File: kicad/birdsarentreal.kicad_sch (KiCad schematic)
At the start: 31 parts, among them J1 Adafruit Coil Jumper, J2 Adafruit Coil Jumper, J3 Adafruit Coil Jumper, J4 Adafruit Coil Jumper, Q2 NMOS, U9 MCP73831-2-OT

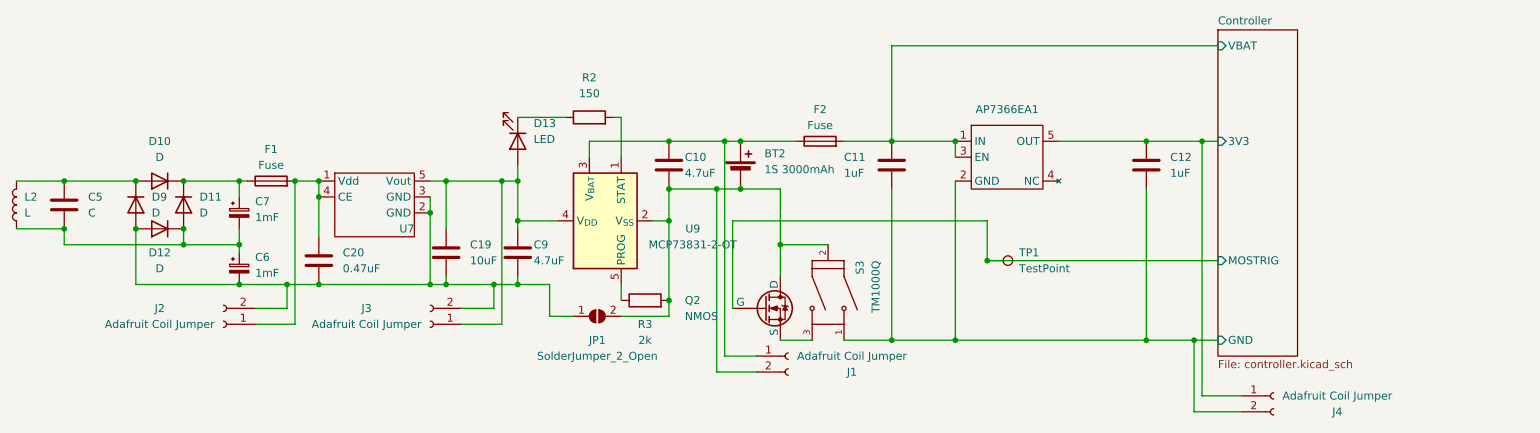
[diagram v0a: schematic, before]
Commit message: First PCB Layout complete
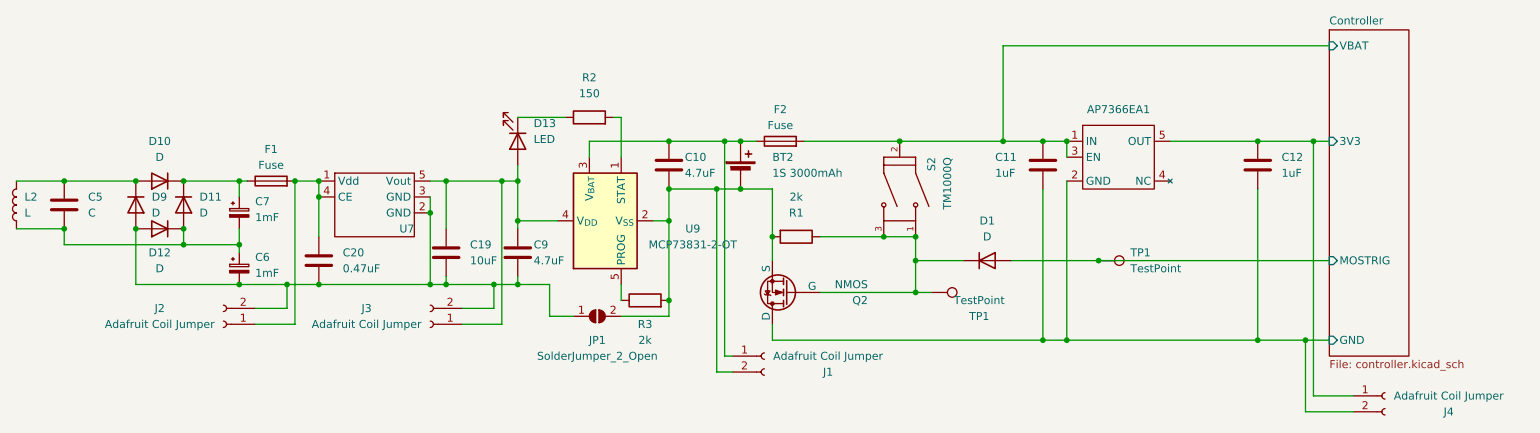
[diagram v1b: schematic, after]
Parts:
- removed S3: TM1000Q, TM1000Q:SW_TM1000Q, symbol TM1000Q:TM1000Q
- added D1: D, Diode_SMD:D_0805_2012Metric_Pad1.15x1.40mm_HandSolder, symbol Device:D
- added R1: 2k, Resistor_SMD:R_0805_2012Metric_Pad1.20x1.40mm_HandSolder, symbol Device:R
- added S2: TM1000Q, TM1000Q:SW_TM1000Q, symbol TM1000Q:TM1000Q
- added TP1: TestPoint, TestPoint:TestPoint_Pad_D2.0mm, symbol Connector:TestPoint
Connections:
- net Controller/GND: now also Q2.1 (D)
- net Controller/MOSTRIG: now also D1.2 (A); no longer Q2.2 (G)
- net Controller/VBAT: now also S2.2
- net at BT2.2 (-), C10.2, J1.2 (Pin_2)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: now also Q2.3 (S), R1.2; no longer Q2.1 (D)
- new net: D1.1 (K), Q2.2 (G), R1.1, S2.1, S2.3, TP1.1
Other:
- moved on the sheet: AP7366EA1, C11, C12, F2, J1, J4, Q2, TP1
